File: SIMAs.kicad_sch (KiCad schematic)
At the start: 1 part, among them U1 mini_esp32

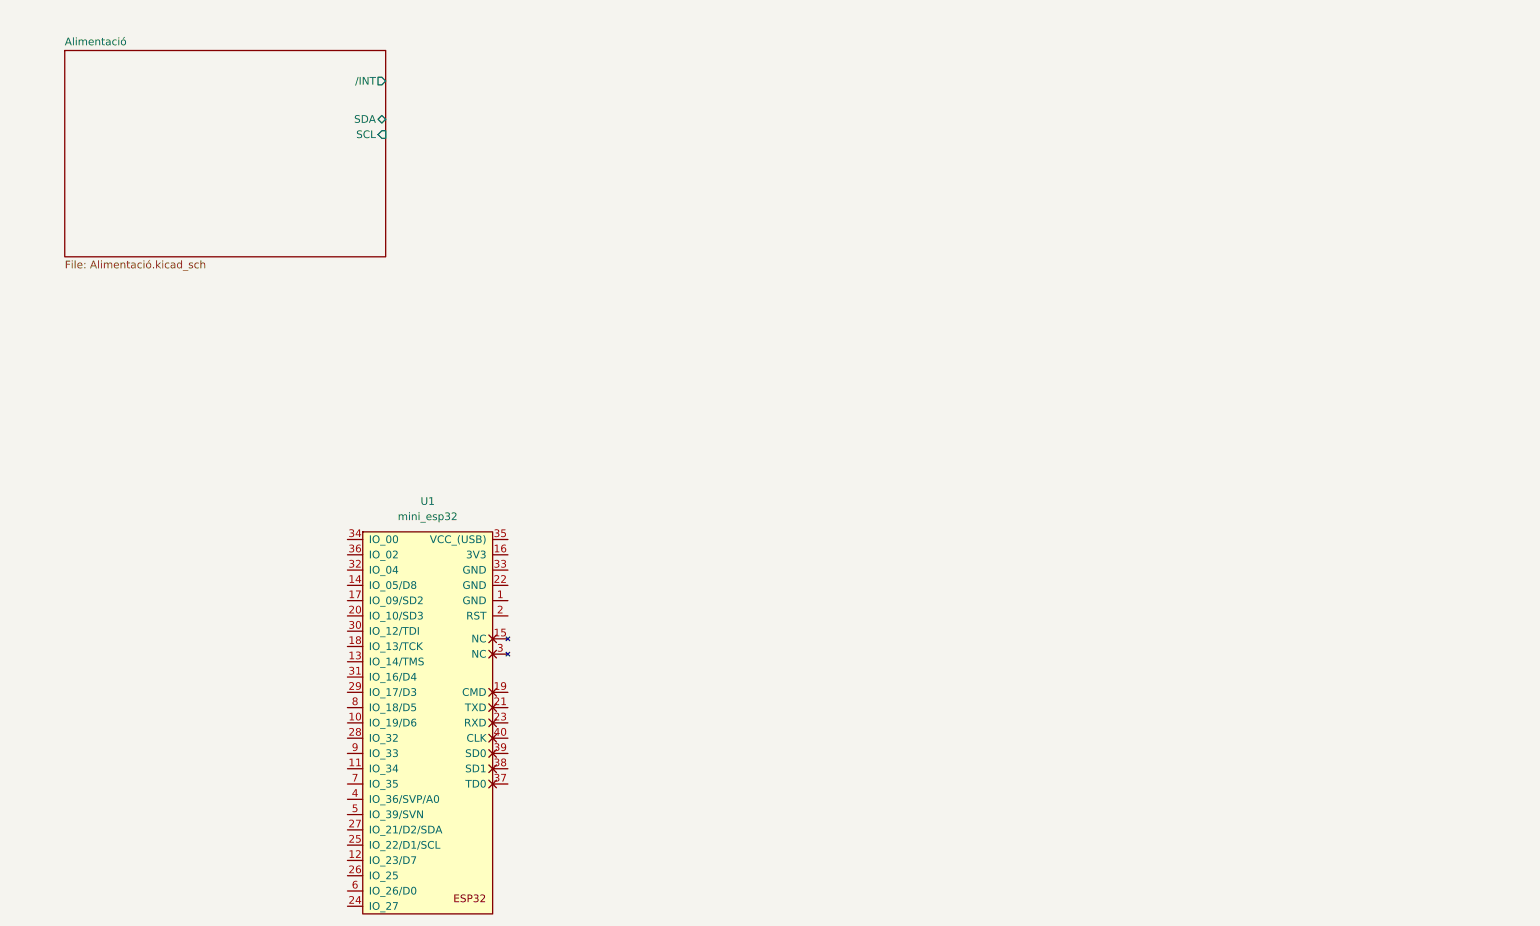
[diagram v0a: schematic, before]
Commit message: Canvi
Algu ha canviat, no recordo
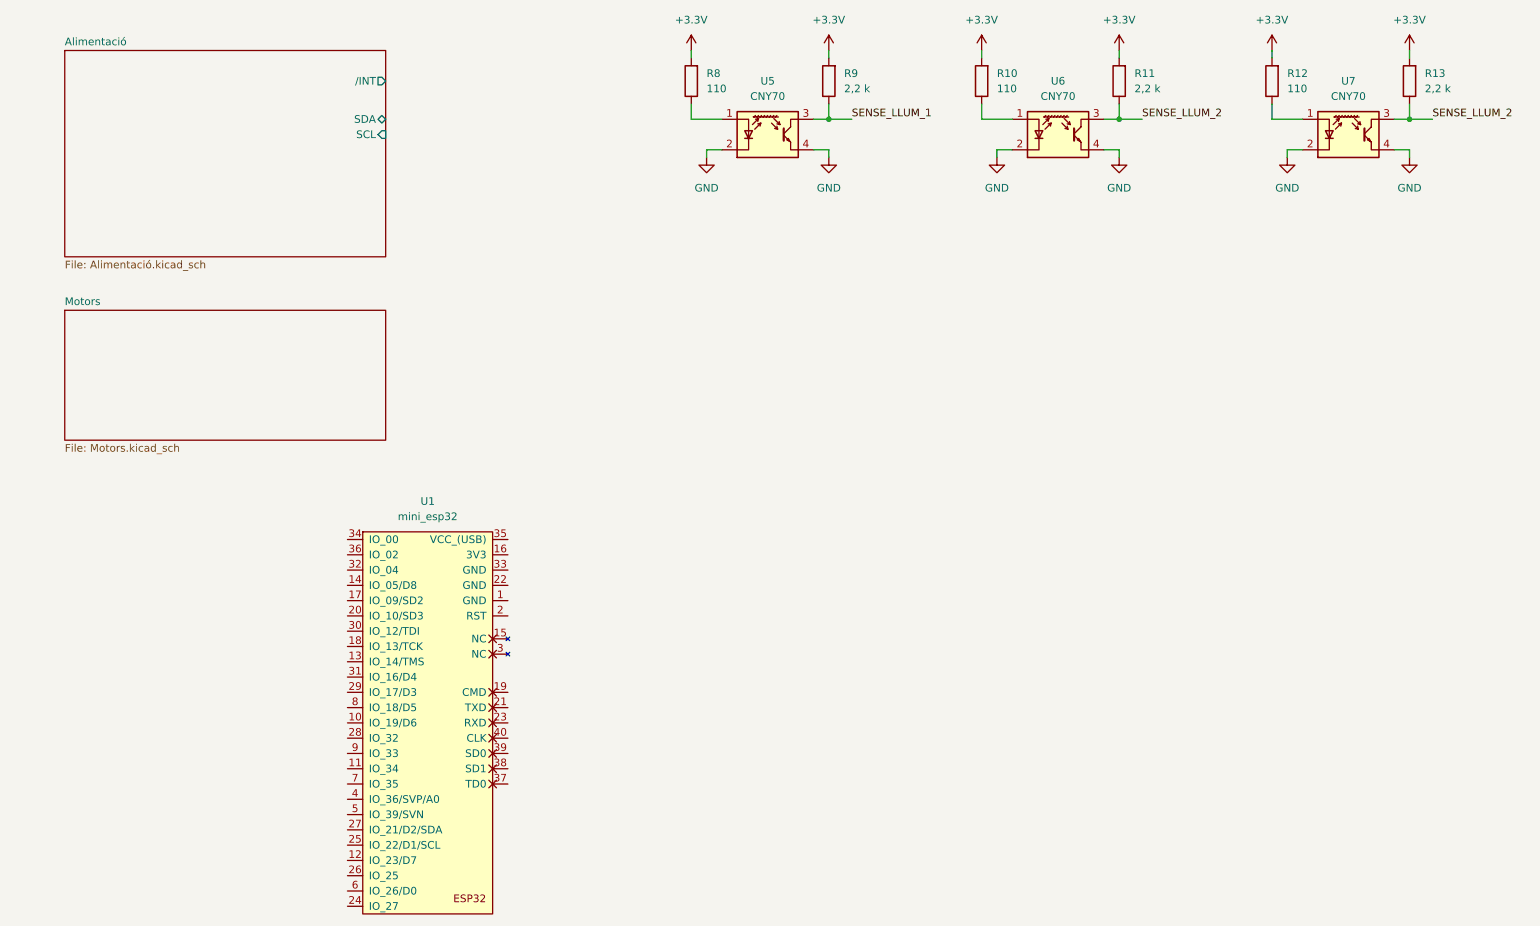
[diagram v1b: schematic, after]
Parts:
- added R10, R12, R8: 110, symbol Device:R
- added R11, R13, R9: 2,2 k, symbol Device:R
- added U5, U6, U7: CNY70, OptoDevice:Vishay_CNY70, symbol Sensor_Proximity:CNY70
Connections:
- new net: R10.1, U6.1 (A)
- new net: R12.1, U7.1 (A)
- new net: R8.1, U5.1 (A)
- new net +3.3V: R10.2, R11.2, R12.2, R13.2, R8.2, R9.2
- new net GND: U5.2 (K), U5.4 (E), U6.2 (K), U6.4 (E), U7.2 (K), U7.4 (E)
- new net SENSE_LLUM_1: R9.1, U5.3 (C)
- new net SENSE_LLUM_2: R11.1, R13.1, U6.3 (C), U7.3 (C)
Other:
- added sheet Motors (Motors.kicad_sch)

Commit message: actualitzar ultrima versio pcb/esquematic
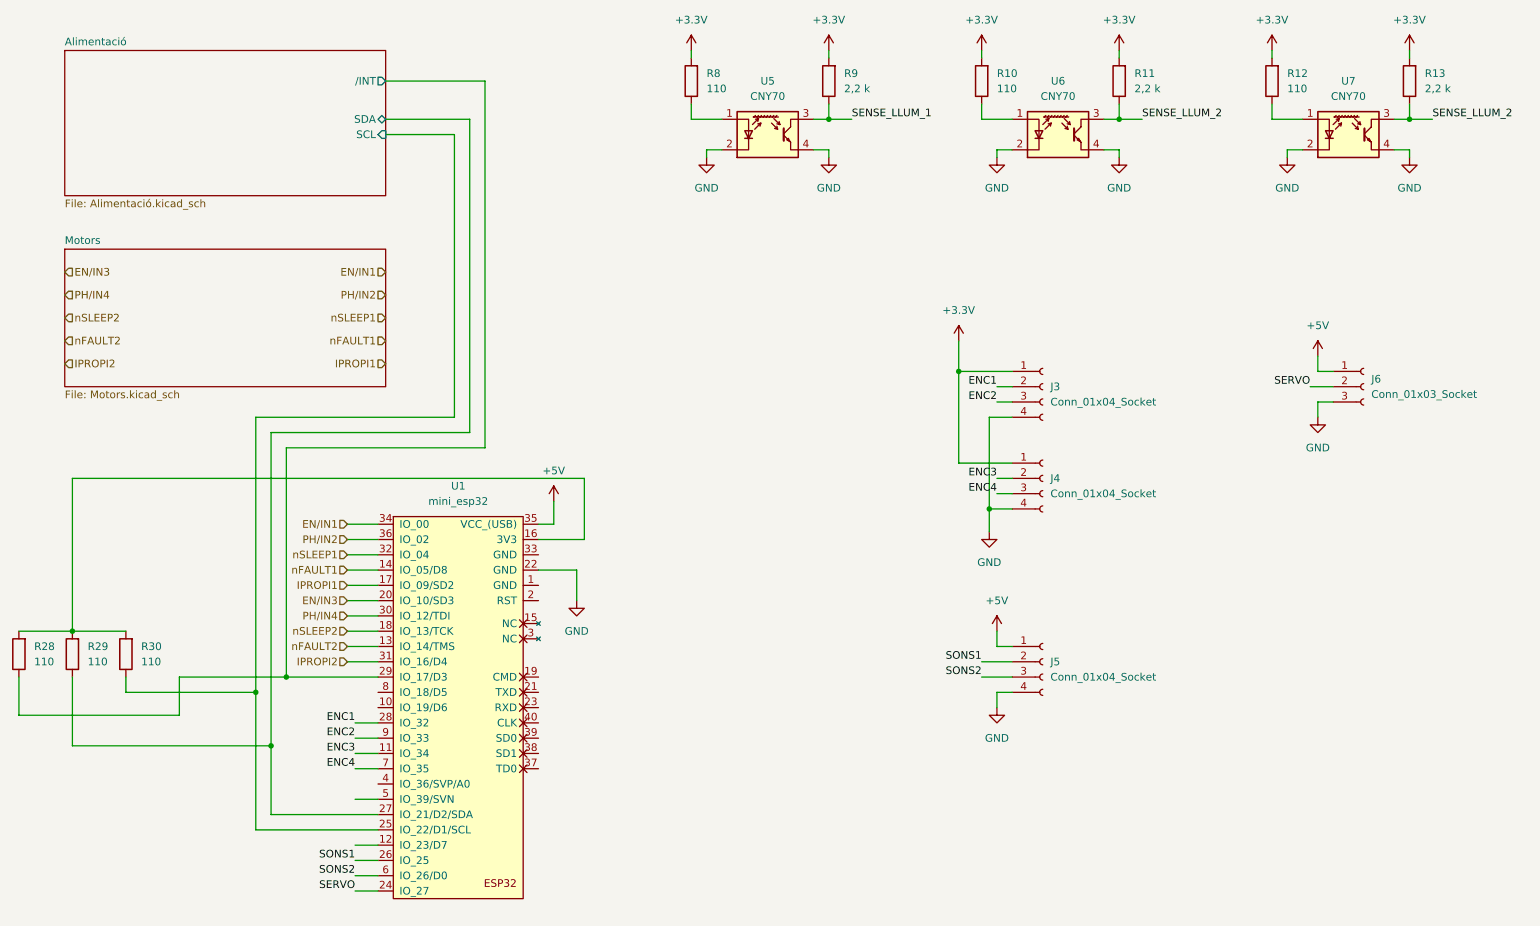
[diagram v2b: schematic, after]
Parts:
- added J3, J4, J5: Conn_01x04_Socket, Connector_JST:JST_PH_B4B-PH-K_1x04_P2.00mm_Vertical, symbol Connector:Conn_01x04_Socket
- added J6: Conn_01x03_Socket, Connector_JST:JST_PH_B3B-PH-K_1x03_P2.00mm_Vertical, symbol Connector:Conn_01x03_Socket
- added R28, R29, R30: 110, Resistor_SMD:R_0201_0603Metric, symbol Device:R
- R10, R11, R12, R13, R8, R9: footprint (none) -> Resistor_SMD:R_0201_0603Metric
- U1: footprint (none) -> ESP32_mini:ESP32_mini
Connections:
- net +3.3V: now also J3.1 (Pin_1), J4.1 (Pin_1)
- net Alimentació/SCL: now also U1.25 (IO_22/D1/SCL), R30.1
- net Alimentació/SDA: now also U1.27 (IO_21/D2/SDA), R29.1
- net Alimentació//INT: now also U1.29 (IO_17/D3), R28.1
- net GND: now also U1.22 (GND), J3.4 (Pin_4), J4.4 (Pin_4), J5.4 (Pin_4), J6.3 (Pin_3)
- net ENC3: now reaches U1.11 (IO_34)
- net ENC3: now also J4.2 (Pin_2)
- net nFAULT2: now reaches U1.13 (IO_14/TMS)
- net nFAULT1: now reaches U1.14 (IO_05/D8)
- net at U1.16 (3V3): now also R28.2, R29.2, R30.2
- net IPROPI1: now reaches U1.17 (IO_09/SD2)
- net nSLEEP2: now reaches U1.18 (IO_13/TCK)
- net EN/IN3: now reaches U1.20 (IO_10/SD3)
- net SERVO: now reaches U1.24 (IO_27)
- net SERVO: now also J6.2 (Pin_2)
- net SONS1: now reaches U1.26 (IO_25)
- net SONS1: now also J5.2 (Pin_2)
- net ENC1: now reaches U1.28 (IO_32)
- net ENC1: now also J3.2 (Pin_2)
- net PH/IN4: now reaches U1.30 (IO_12/TDI)
- net IPROPI2: now reaches U1.31 (IO_16/D4)
- net nSLEEP1: now reaches U1.32 (IO_04)
- net EN/IN1: now reaches U1.34 (IO_00)
- net +5V: now reaches U1.35 (VCC_(USB))
- net +5V: now also J5.1 (Pin_1), J6.1 (Pin_1)
- net PH/IN2: now reaches U1.36 (IO_02)
- net SONS2: now reaches U1.6 (IO_26/D0)
- net SONS2: now also J5.3 (Pin_3)
- net ENC4: now reaches U1.7 (IO_35)
- net ENC4: now also J4.3 (Pin_3)
- net ENC2: now reaches U1.9 (IO_33)
- net ENC2: now also J3.3 (Pin_3)
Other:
- moved on the sheet: U1
